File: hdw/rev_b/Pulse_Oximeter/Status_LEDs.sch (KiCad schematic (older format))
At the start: 20 parts, among them U1901 74LVC1G06, U1902 74LVC1G06, U1903 74LVC1G06, U1904 74LVC1G06

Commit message: lots of rev b changes
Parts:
- removed U1901, U1902, U1903, U1904: 74LVC1G06, TO_SOT_Packages_SMD:SOT-353_SC-70-5, symbol Custom_Library:74LVC1G06_Power
- added U? (x4): 74LVC1G97, Package_TO_SOT_SMD:SOT-363_SC-70-6, symbol Custom_Library:74LVC1G97_Power_NOT
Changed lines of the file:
@@
 	1    0    0    -1
 $EndComp
+Text GLabel 1770 4220 0    50   Input ~ 0
+Error_LED
 $Comp
-L Custom_Library:74LVC1G06_Power U?
-U 1 1 5EBB3661
+L Custom_Library:74LVC1G97_Power_NOT U?
+U 1 1 5FDC38B1
 P 2400 2220
-AR Path="/5EAE4ADE/5EBB3661" Ref="U?"  Part="1"
-AR Path="/5EAE4AE4/5EBB3661" Ref="U1901"  Part="1"
-F 0 "U1901" H 2500 2370 50  0000 L CNN
-F 1 "74LVC1G06" H 2500 2120 50  0000 L CNN
-F 2 "TO_SOT_Packages_SMD:SOT-353_SC-70-5" H 2400 2270 50  0001 C CNN
-F 3 "http://www.ti.com/lit/ds/symlink/sn74lvc1g06.pdf" H 2400 2220 50  0001 C CNN
-F 4 "296-8484-1-ND" H 2400 2220 50  0001 C CNN "Digi-Key PN"
+F 0 "U?" H 2460 2370 50  0000 L CNN
+F 1 "74LVC1G97" H 2460 2070 50  0000 L CNN
+F 2 "Package_TO_SOT_SMD:SOT-363_SC-70-6" H 2450 2220 50  0001 C CNN
+F 3 "http://www.ti.com/lit/ds/symlink/sn74lvc1g97.pdf" H 2450 2220 50  0001 C CNN
 	1    2400 2220
 	1    0    0    -1
 $EndComp
 $Comp
-L Custom_Library:74LVC1G06_Power U?
-U 1 1 5EBB3BCA
+L Custom_Library:74LVC1G97_Power_NOT U?
+U 1 1 5FDC4D56
 P 4400 2220
-AR Path="/5EAE4ADE/5EBB3BCA" Ref="U?"  Part="1"
-AR Path="/5EAE4AE4/5EBB3BCA" Ref="U1903"  Part="1"
-F 0 "U1903" H 4500 2370 50  0000 L CNN
-F 1 "74LVC1G06" H 4500 2120 50  0000 L CNN
-F 2 "TO_SOT_Packages_SMD:SOT-353_SC-70-5" H 4400 2270 50  0001 C CNN
-F 3 "http://www.ti.com/lit/ds/symlink/sn74lvc1g06.pdf" H 4400 2220 50  0001 C CNN
-F 4 "296-8484-1-ND" H 4400 2220 50  0001 C CNN "Digi-Key PN"
+F 0 "U?" H 4460 2370 50  0000 L CNN
+F 1 "74LVC1G97" H 4460 2070 50  0000 L CNN
+F 2 "Package_TO_SOT_SMD:SOT-363_SC-70-6" H 4450 2220 50  0001 C CNN
+F 3 "http://www.ti.com/lit/ds/symlink/sn74lvc1g97.pdf" H 4450 2220 50  0001 C CNN
 	1    4400 2220
 	1    0    0    -1
 $EndComp
 $Comp
-L Custom_Library:74LVC1G06_Power U?
-U 1 1 5EBB56C7
+L Custom_Library:74LVC1G97_Power_NOT U?
+U 1 1 5FDC5735
 P 4400 4220
-AR Path="/5EAE4ADE/5EBB56C7" Ref="U?"  Part="1"
-AR Path="/5EAE4AE4/5EBB56C7" Ref="U1904"  Part="1"
-F 0 "U1904" H 4500 4370 50  0000 L CNN
-F 1 "74LVC1G06" H 4500 4120 50  0000 L CNN
-F 2 "TO_SOT_Packages_SMD:SOT-353_SC-70-5" H 4400 4270 50  0001 C CNN
-F 3 "http://www.ti.com/lit/ds/symlink/sn74lvc1g06.pdf" H 4400 4220 50  0001 C CNN
-F 4 "296-8484-1-ND" H 4400 4220 50  0001 C CNN "Digi-Key PN"
+F 0 "U?" H 4460 4370 50  0000 L CNN
+F 1 "74LVC1G97" H 4460 4070 50  0000 L CNN
+F 2 "Package_TO_SOT_SMD:SOT-363_SC-70-6" H 4450 4220 50  0001 C CNN
+F 3 "http://www.ti.com/lit/ds/symlink/sn74lvc1g97.pdf" H 4450 4220 50  0001 C CNN
 	1    4400 4220
 	1    0    0    -1
 $EndComp
 $Comp
-L Custom_Library:74LVC1G06_Power U?
-U 1 1 5EBB6CE5
+L Custom_Library:74LVC1G97_Power_NOT U?
+U 1 1 5FDC5DDB
 P 2400 4220
-AR Path="/5EAE4ADE/5EBB6CE5" Ref="U?"  Part="1"
-AR Path="/5EAE4AE4/5EBB6CE5" Ref="U1902"  Part="1"
-F 0 "U1902" H 2500 4370 50  0000 L CNN
-F 1 "74LVC1G06" H 2500 4120 50  0000 L CNN
-F 2 "TO_SOT_Packages_SMD:SOT-353_SC-70-5" H 2400 4270 50  0001 C CNN
-F 3 "http://www.ti.com/lit/ds/symlink/sn74lvc1g06.pdf" H 2400 4220 50  0001 C CNN
-F 4 "296-8484-1-ND" H 2400 4220 50  0001 C CNN "Digi-Key PN"
+F 0 "U?" H 2460 4370 50  0000 L CNN
+F 1 "74LVC1G97" H 2460 4070 50  0000 L CNN
+F 2 "Package_TO_SOT_SMD:SOT-363_SC-70-6" H 2450 4220 50  0001 C CNN
+F 3 "http://www.ti.com/lit/ds/symlink/sn74lvc1g97.pdf" H 2450 4220 50  0001 C CNN
 	1    2400 4220
 	1    0    0    -1
 $EndComp
-Text GLabel 1770 4220 0    50   Input ~ 0
-Error_LED
 $EndSCHEMATC

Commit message: changed all passives to 0402, cleared digikey pns
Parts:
- C1901, C1902, C1903, C1904: Digi-Key PN 490-10701-1-ND -> (none)
- R1901, R1902, R1905, R1906: Digi-Key PN RMCF0402FT10K0CT-ND -> (none)
- R1903, R1904, R1907, R1908: Digi-Key PN 541-1.00KLCT-ND -> (none)
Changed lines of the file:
@@
 F 2 "Capacitors_SMD:C_0402" H 2328 1380 50  0001 C CNN
 F 3 "" H 2315 1630 50  0001 C CNN
-F 4 "490-10701-1-ND" H 2715 2030 60  0001 C CNN "Digi-Key PN"
+F 4 "" H 2715 2030 60  0001 C CNN "Digi-Key PN"
 F 5 "0402" H 2140 1630 50  0000 R CNN "display_footprint"
 F 6 "50V" H 2140 1530 50  0000 R CNN "Voltage"
@@
 F 5 "1%" H 3040 1650 50  0000 L CNN "Tolerance"
 F 6 "1/16W" H 3040 1580 50  0000 L CNN "Wattage"
-F 7 "541-1.00KLCT-ND" H 3270 2050 60  0001 C CNN "Digi-Key PN"
+F 7 "" H 3270 2050 60  0001 C CNN "Digi-Key PN"
 	1    2970 1650
 	-1   0    0    -1
@@
 F 5 "1%" H 1920 2450 50  0000 L CNN "Tolerance"
 F 6 "1/16W" H 1920 2380 50  0000 L CNN "Wattage"
-F 7 "RMCF0402FT10K0CT-ND" H 1850 2450 50  0001 C CNN "Digi-Key PN"
+F 7 "" H 1850 2450 50  0001 C CNN "Digi-Key PN"
 	1    1850 2450
 	-1   0    0    -1
@@
 F 2 "Capacitors_SMD:C_0402" H 4328 1380 50  0001 C CNN
 F 3 "" H 4315 1630 50  0001 C CNN
-F 4 "490-10701-1-ND" H 4715 2030 60  0001 C CNN "Digi-Key PN"
+F 4 "" H 4715 2030 60  0001 C CNN "Digi-Key PN"
 F 5 "0402" H 4140 1630 50  0000 R CNN "display_footprint"
 F 6 "50V" H 4140 1530 50  0000 R CNN "Voltage"
@@
 F 5 "1%" H 5040 1650 50  0000 L CNN "Tolerance"
 F 6 "1/16W" H 5040 1580 50  0000 L CNN "Wattage"
-F 7 "541-1.00KLCT-ND" H 5270 2050 60  0001 C CNN "Digi-Key PN"
+F 7 "" H 5270 2050 60  0001 C CNN "Digi-Key PN"
 	1    4970 1650
 	-1   0    0    -1
@@
 F 5 "1%" H 3920 1990 50  0000 L CNN "Tolerance"
 F 6 "1/16W" H 3920 1920 50  0000 L CNN "Wattage"
-F 7 "RMCF0402FT10K0CT-ND" H 3850 1990 50  0001 C CNN "Digi-Key PN"
+F 7 "" H 3850 1990 50  0001 C CNN "Digi-Key PN"
 	1    3850 1990
 	-1   0    0    -1
@@
 F 2 "Capacitors_SMD:C_0402" H 4328 3380 50  0001 C CNN
 F 3 "" H 4315 3630 50  0001 C CNN
-F 4 "490-10701-1-ND" H 4715 4030 60  0001 C CNN "Digi-Key PN"
+F 4 "" H 4715 4030 60  0001 C CNN "Digi-Key PN"
 F 5 "0402" H 4140 3630 50  0000 R CNN "display_footprint"
 F 6 "50V" H 4140 3530 50  0000 R CNN "Voltage"
@@
 F 5 "1%" H 5040 3650 50  0000 L CNN "Tolerance"
 F 6 "1/16W" H 5040 3580 50  0000 L CNN "Wattage"
-F 7 "541-1.00KLCT-ND" H 5270 4050 60  0001 C CNN "Digi-Key PN"
+F 7 "" H 5270 4050 60  0001 C CNN "Digi-Key PN"
 	1    4970 3650
 	-1   0    0    -1
@@
 F 5 "1%" H 3920 4450 50  0000 L CNN "Tolerance"
 F 6 "1/16W" H 3920 4380 50  0000 L CNN "Wattage"
-F 7 "RMCF0402FT10K0CT-ND" H 3850 4450 50  0001 C CNN "Digi-Key PN"
+F 7 "" H 3850 4450 50  0001 C CNN "Digi-Key PN"
 	1    3850 4450
 	-1   0    0    -1
@@
 F 2 "Capacitors_SMD:C_0402" H 2328 3380 50  0001 C CNN
 F 3 "" H 2315 3630 50  0001 C CNN
-F 4 "490-10701-1-ND" H 2715 4030 60  0001 C CNN "Digi-Key PN"
+F 4 "" H 2715 4030 60  0001 C CNN "Digi-Key PN"
 F 5 "0402" H 2140 3630 50  0000 R CNN "display_footprint"
 F 6 "50V" H 2140 3530 50  0000 R CNN "Voltage"
@@
 F 5 "1%" H 3040 3650 50  0000 L CNN "Tolerance"
 F 6 "1/16W" H 3040 3580 50  0000 L CNN "Wattage"
-F 7 "541-1.00KLCT-ND" H 3270 4050 60  0001 C CNN "Digi-Key PN"
+F 7 "" H 3270 4050 60  0001 C CNN "Digi-Key PN"
 	1    2970 3650
 	-1   0    0    -1
@@
 F 5 "1%" H 1920 4450 50  0000 L CNN "Tolerance"
 F 6 "1/16W" H 1920 4380 50  0000 L CNN "Wattage"
-F 7 "RMCF0402FT10K0CT-ND" H 1850 4450 50  0001 C CNN "Digi-Key PN"
+F 7 "" H 1850 4450 50  0001 C CNN "Digi-Key PN"
 	1    1850 4450
 	-1   0    0    -1

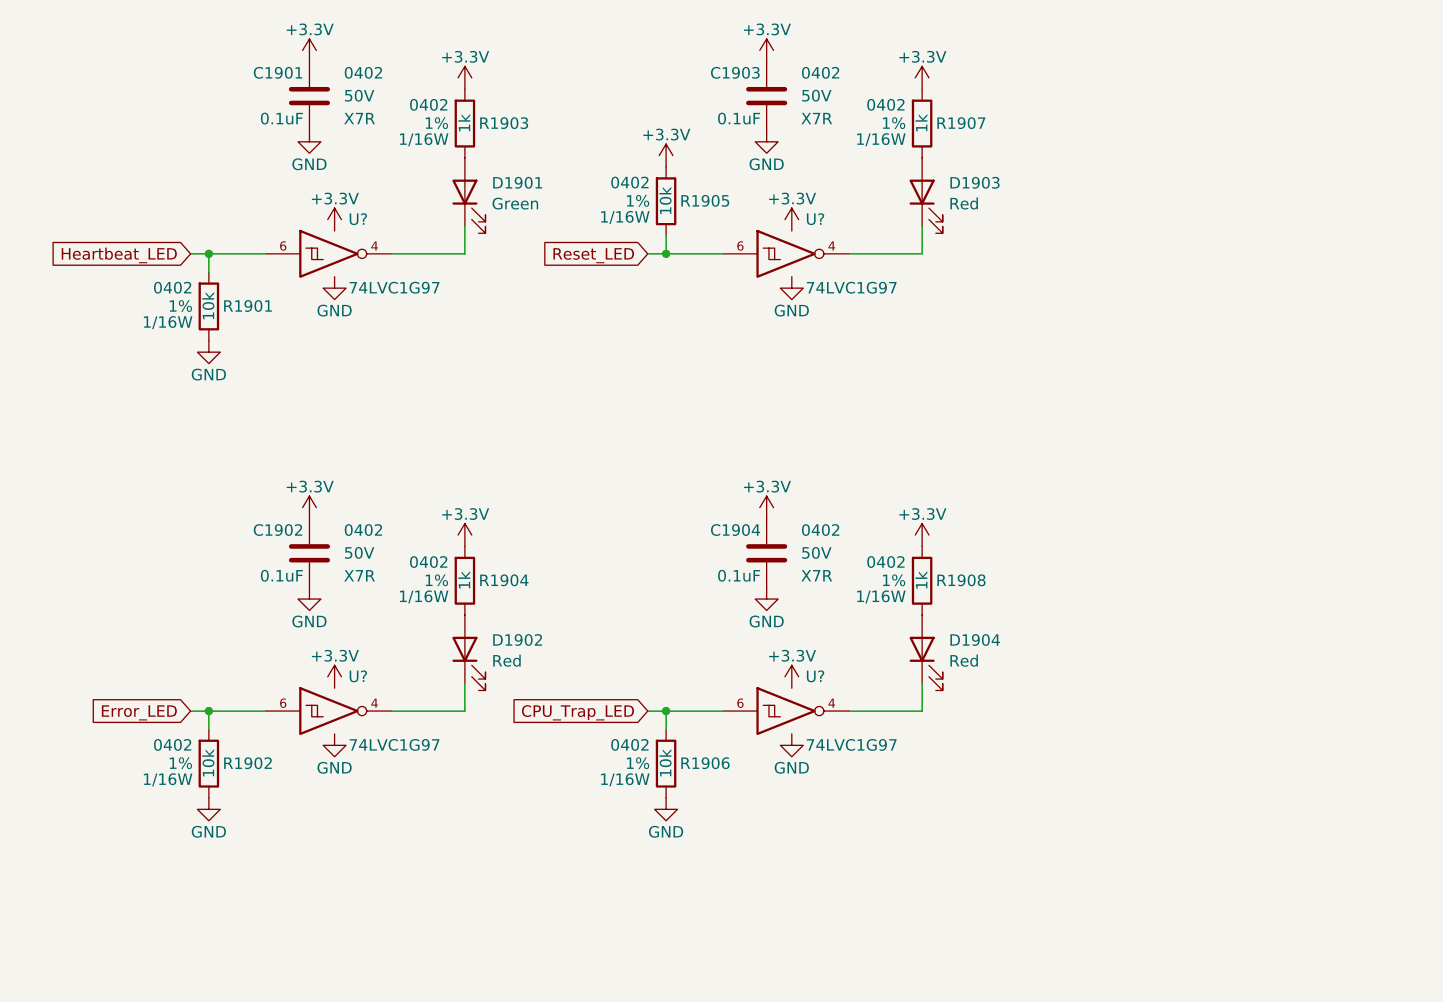
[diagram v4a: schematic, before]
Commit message: few little tweaks
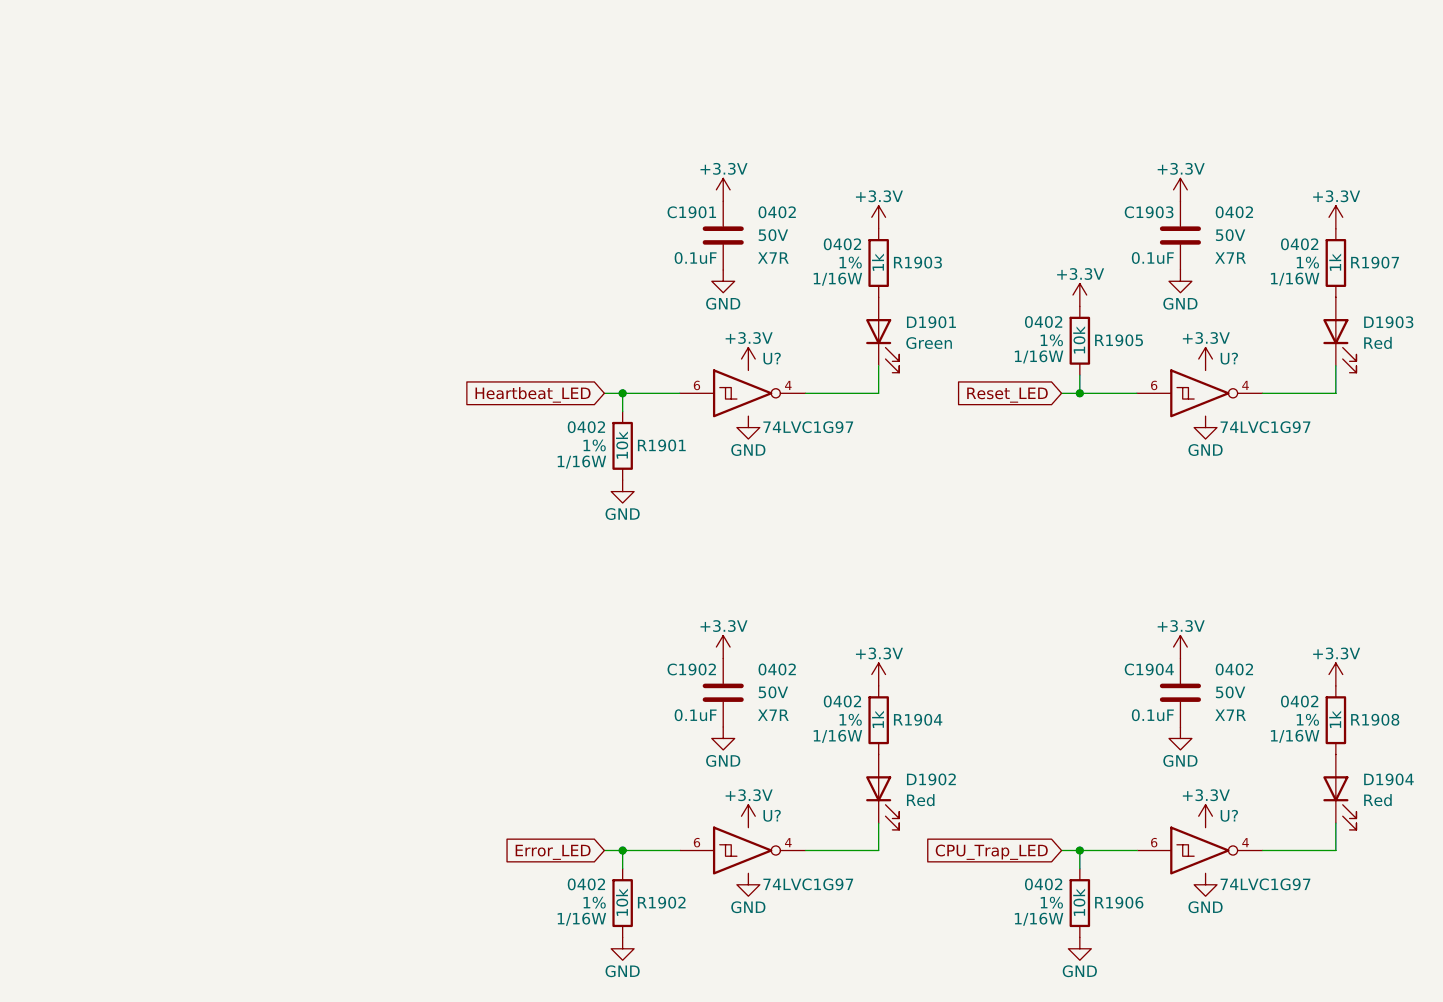
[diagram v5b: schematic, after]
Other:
- moved on the sheet: C1901, C1902, C1903, C1904, D1901, D1902, D1903, D1904, R1901, R1902, R1903, R1904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

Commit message: annotated schematic
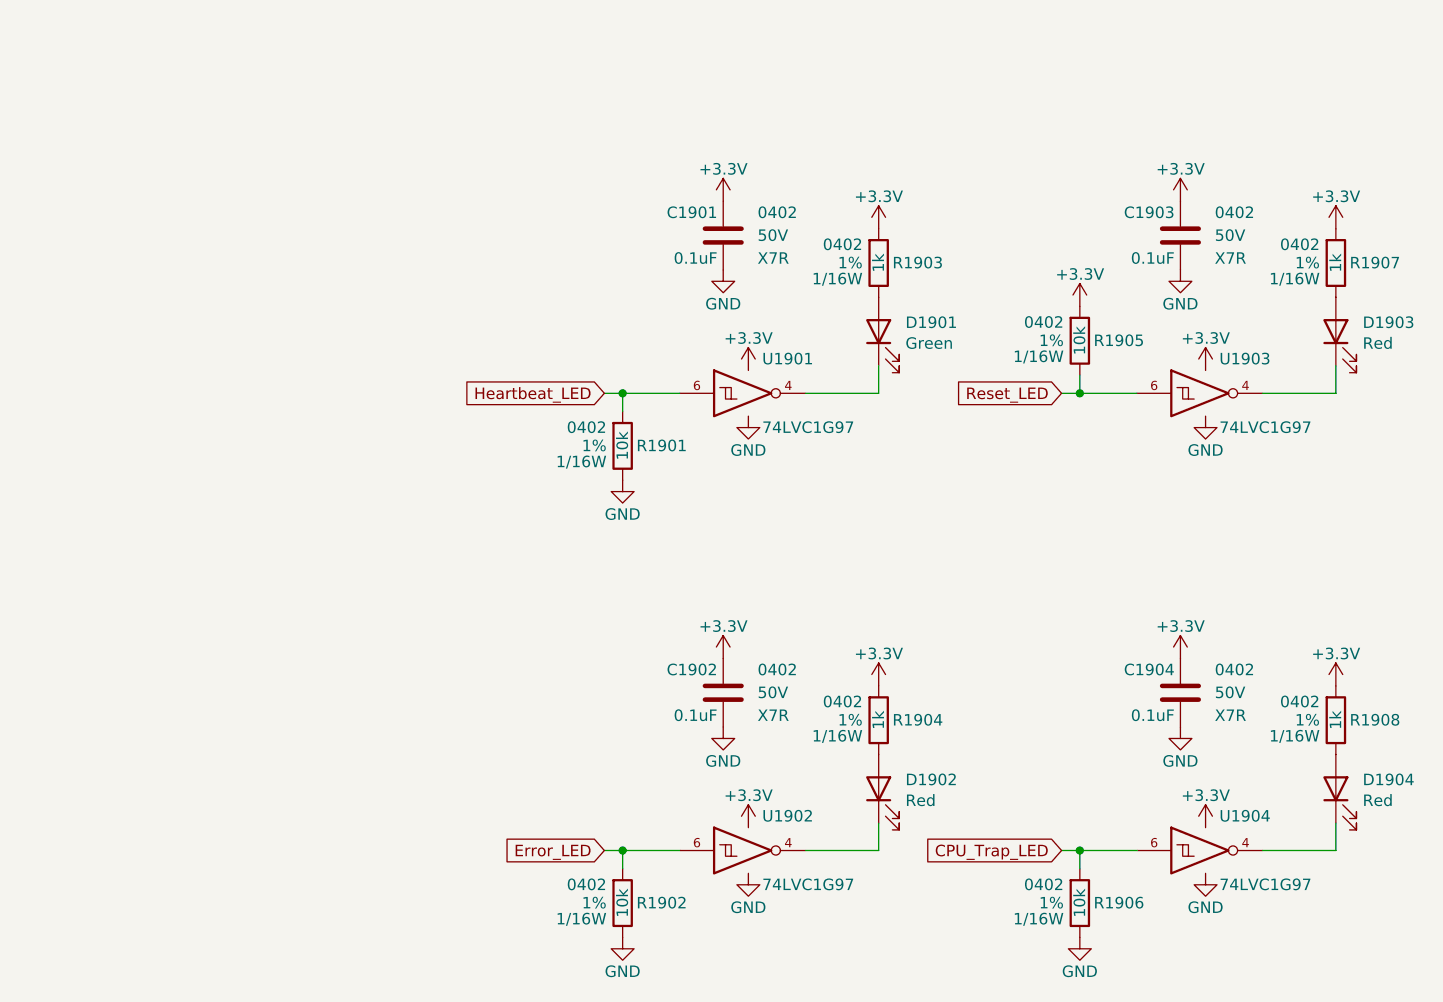
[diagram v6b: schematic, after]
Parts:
- U1901, U1902, U1903, U1904: renamed from U?; Digi-Key PN (none) -> 296-SN74LVC1G97DCK3CT-ND
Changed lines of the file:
@@
 Error_LED
 $Comp
-L Custom_Library:74LVC1G97_Power_NOT U?
+L Custom_Library:74LVC1G97_Power_NOT U1901
 U 1 1 5FDC38B1
 P 4210 2830
-F 0 "U?" H 4270 2980 50  0000 L CNN
+F 0 "U1901" H 4270 2980 50  0000 L CNN
 F 1 "74LVC1G97" H 4270 2680 50  0000 L CNN
 F 2 "Package_TO_SOT_SMD:SOT-363_SC-70-6" H 4260 2830 50  0001 C CNN
 F 3 "http://www.ti.com/lit/ds/symlink/sn74lvc1g97.pdf" H 4260 2830 50  0001 C CNN
+F 4 "296-SN74LVC1G97DCK3CT-ND" H 4210 2830 50  0001 C CNN "Digi-Key PN"
 	1    4210 2830
 	1    0    0    -1
 $EndComp
 $Comp
-L Custom_Library:74LVC1G97_Power_NOT U?
+L Custom_Library:74LVC1G97_Power_NOT U1903
 U 1 1 5FDC4D56
 P 6210 2830
-F 0 "U?" H 6270 2980 50  0000 L CNN
+F 0 "U1903" H 6270 2980 50  0000 L CNN
 F 1 "74LVC1G97" H 6270 2680 50  0000 L CNN
 F 2 "Package_TO_SOT_SMD:SOT-363_SC-70-6" H 6260 2830 50  0001 C CNN
 F 3 "http://www.ti.com/lit/ds/symlink/sn74lvc1g97.pdf" H 6260 2830 50  0001 C CNN
+F 4 "296-SN74LVC1G97DCK3CT-ND" H 6210 2830 50  0001 C CNN "Digi-Key PN"
 	1    6210 2830
 	1    0    0    -1
 $EndComp
 $Comp
-L Custom_Library:74LVC1G97_Power_NOT U?
+L Custom_Library:74LVC1G97_Power_NOT U1904
 U 1 1 5FDC5735
 P 6210 4830
-F 0 "U?" H 6270 4980 50  0000 L CNN
+F 0 "U1904" H 6270 4980 50  0000 L CNN
 F 1 "74LVC1G97" H 6270 4680 50  0000 L CNN
 F 2 "Package_TO_SOT_SMD:SOT-363_SC-70-6" H 6260 4830 50  0001 C CNN
 F 3 "http://www.ti.com/lit/ds/symlink/sn74lvc1g97.pdf" H 6260 4830 50  0001 C CNN
+F 4 "296-SN74LVC1G97DCK3CT-ND" H 6210 4830 50  0001 C CNN "Digi-Key PN"
 	1    6210 4830
 	1    0    0    -1
 $EndComp
 $Comp
-L Custom_Library:74LVC1G97_Power_NOT U?
+L Custom_Library:74LVC1G97_Power_NOT U1902
 U 1 1 5FDC5DDB
 P 4210 4830
-F 0 "U?" H 4270 4980 50  0000 L CNN
+F 0 "U1902" H 4270 4980 50  0000 L CNN
 F 1 "74LVC1G97" H 4270 4680 50  0000 L CNN
 F 2 "Package_TO_SOT_SMD:SOT-363_SC-70-6" H 4260 4830 50  0001 C CNN
 F 3 "http://www.ti.com/lit/ds/symlink/sn74lvc1g97.pdf" H 4260 4830 50  0001 C CNN
+F 4 "296-SN74LVC1G97DCK3CT-ND" H 4210 4830 50  0001 C CNN "Digi-Key PN"
 	1    4210 4830
 	1    0    0    -1
